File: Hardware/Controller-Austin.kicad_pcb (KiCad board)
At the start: 2 copper layers, 34 x 34 mm, 12 parts, among them J2 Conn_01x04_Male, J3 Conn_01x02_Male, J4 Conn_01x02_Male, J5 Conn_01x02_Male, J6 Conn_01x02_Male, J9 Conn_01x04_MountingPin

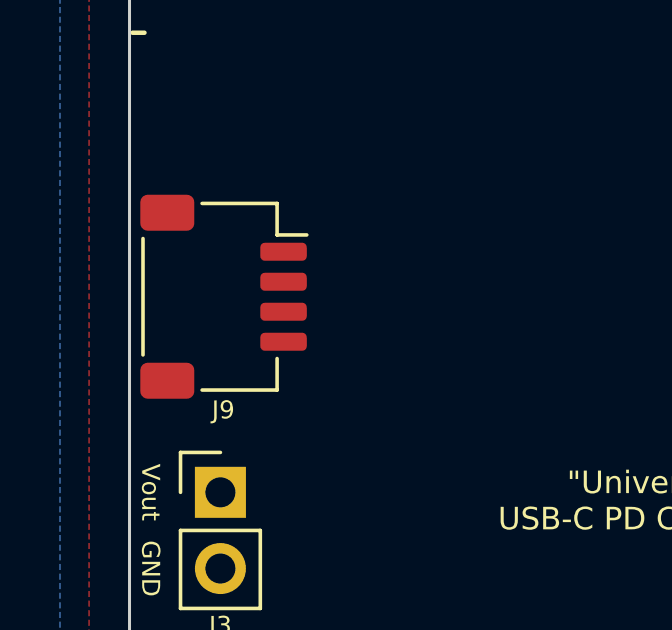
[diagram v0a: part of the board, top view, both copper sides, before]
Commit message: starting on controller boards
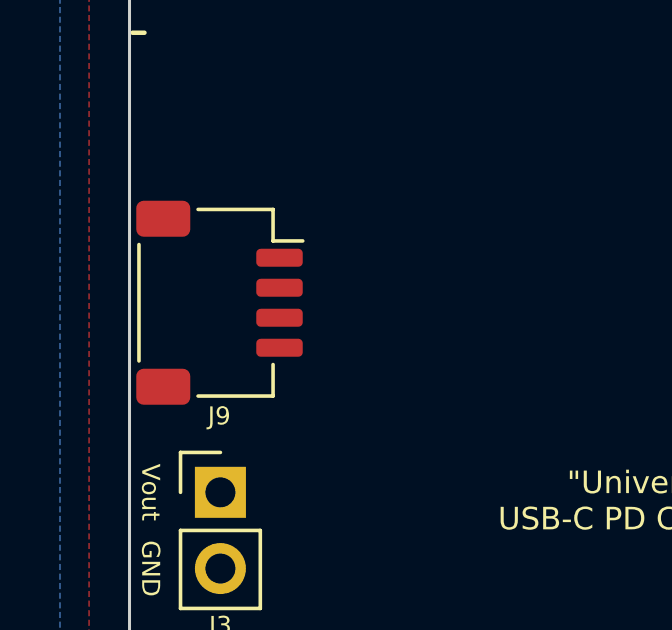
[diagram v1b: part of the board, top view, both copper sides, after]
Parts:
- moved J9 0.24 mm to (86.0, 87.0)
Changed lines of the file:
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@@
   )
   (footprint "Tinker:JST_SH_SM04B-SRSS-TB_1x04-1MP_P1.00mm_Horizontal" (layer "F.Cu")
-    (at 86.13441 86.8 -90)
+    (at 86 87 -90)
     (descr "JST SH series connector, SM04B-SRSS-TB (http://www.jst-mfg.com/product/pdf/eng/eSH.pdf), generated with kicad-footprint-generator")
     (tags "connector JST SH top entry")
@@
     (pad "2" thru_hole oval (at 0 2.54) (size 1.7 1.7) (drill 1) (layers *.Cu *.Mask)
       (net 6 "GND") (pinfunction "Pin_2") (pintype "passive"))
-    (model "${KICAD6_3DMODEL_DIR}/Connector_PinHeader_2.54mm.3dshapes/PinHeader_1x02_P2.54mm_Vertical.wrl"
+    (model "${KICAD6_3DMODEL_DIR}/Connector_PinHeader_2.54mm.3dshapes/PinHeader_1x02_P2.54mm_Vertical.wrl" hide
       (offset (xyz 0 0 0))
       (scale (xyz 1 1 1))
@@
     (pad "2" thru_hole oval (at 0 2.54) (size 1.7 1.7) (drill 1) (layers *.Cu *.Mask)
       (net 6 "GND") (pinfunction "Pin_2") (pintype "passive"))
-    (model "${KICAD6_3DMODEL_DIR}/Connector_PinHeader_2.54mm.3dshapes/PinHeader_1x02_P2.54mm_Vertical.wrl"
+    (model "${KICAD6_3DMODEL_DIR}/Connector_PinHeader_2.54mm.3dshapes/PinHeader_1x02_P2.54mm_Vertical.wrl" hide
       (offset (xyz 0 0 0))
       (scale (xyz 1 1 1))
@@
     (pad "2" thru_hole oval (at 0 2.54) (size 1.7 1.7) (drill 1) (layers *.Cu *.Mask)
       (net 6 "GND") (pinfunction "Pin_2") (pintype "passive"))
-    (model "${KICAD6_3DMODEL_DIR}/Connector_PinHeader_2.54mm.3dshapes/PinHeader_1x02_P2.54mm_Vertical.wrl"
+    (model "${KICAD6_3DMODEL_DIR}/Connector_PinHeader_2.54mm.3dshapes/PinHeader_1x02_P2.54mm_Vertical.wrl" hide
       (offset (xyz 0 0 0))
       (scale (xyz 1 1 1))
@@
     (pad "2" thru_hole oval (at 0 2.54) (size 1.7 1.7) (drill 1) (layers *.Cu *.Mask)
       (net 6 "GND") (pinfunction "Pin_2") (pintype "passive"))
-    (model "${KICAD6_3DMODEL_DIR}/Connector_PinHeader_2.54mm.3dshapes/PinHeader_1x02_P2.54mm_Vertical.wrl"
+    (model "${KICAD6_3DMODEL_DIR}/Connector_PinHeader_2.54mm.3dshapes/PinHeader_1x02_P2.54mm_Vertical.wrl" hide
       (offset (xyz 0 0 0))
       (scale (xyz 1 1 1))
@@
     (pad "4" thru_hole oval (at 0 7.62 270) (size 1.7 1.7) (drill 1) (layers *.Cu *.Mask)
       (net 6 "GND") (pinfunction "Pin_4") (pintype "passive"))
-    (model "${KICAD6_3DMODEL_DIR}/Connector_PinHeader_2.54mm.3dshapes/PinHeader_1x04_P2.54mm_Vertical.wrl"
+    (model "${KICAD6_3DMODEL_DIR}/Connector_PinHeader_2.54mm.3dshapes/PinHeader_1x04_P2.54mm_Vertical.wrl" hide
       (offset (xyz 0 0 0))
       (scale (xyz 1 1 1))
